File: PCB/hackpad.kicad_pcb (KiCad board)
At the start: 2 copper layers, 93.8 x 82 mm, 36 parts, among them SW11 SW_Push, SW12 SW_Push, SW13 SW_Push, SW14 SW_Push, SW15 SW_Push, SW16 SW_Push, SW17 SW_Push, SW18 SW_Push, SW19 SW_Push, SW4 RotaryEncoder_Switch, U1 MOUDLE-SEEEDUINO-XIAO, U2 ER_OLEDM0.91_1x-I2C

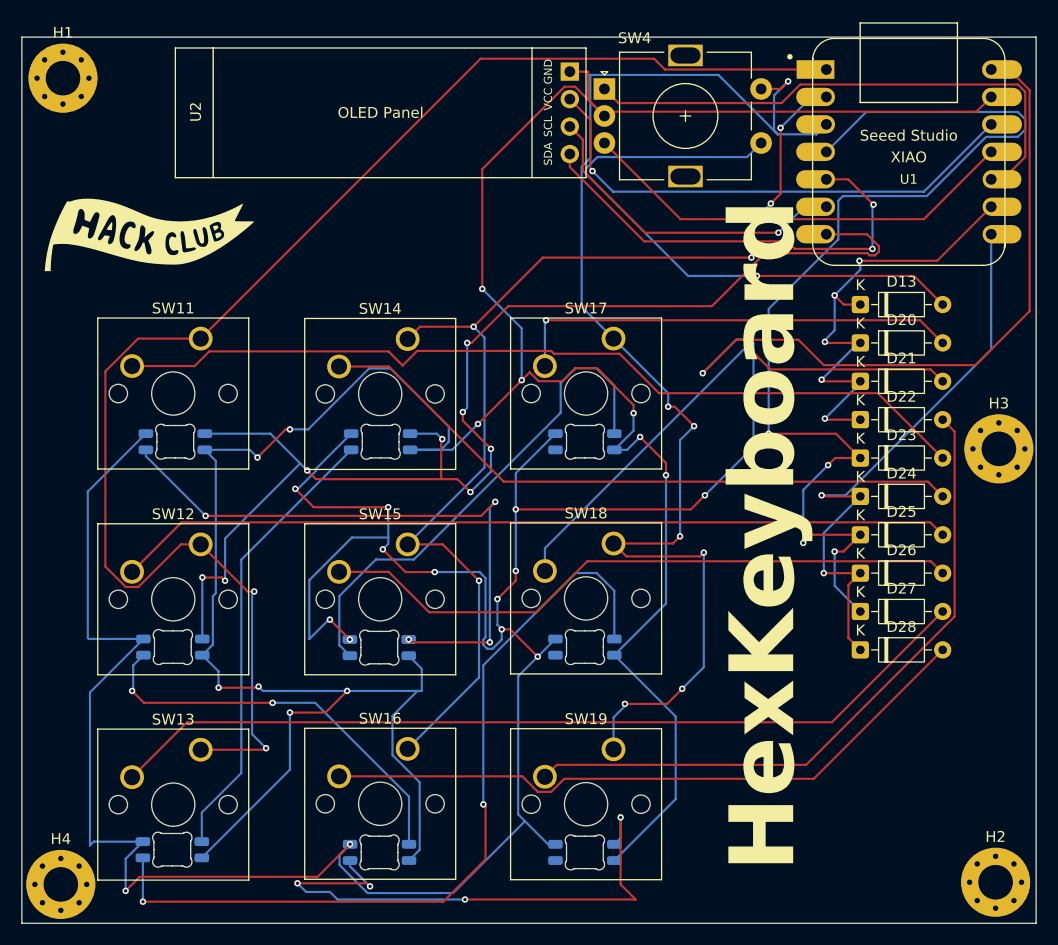
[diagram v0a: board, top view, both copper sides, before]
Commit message: PCB Update
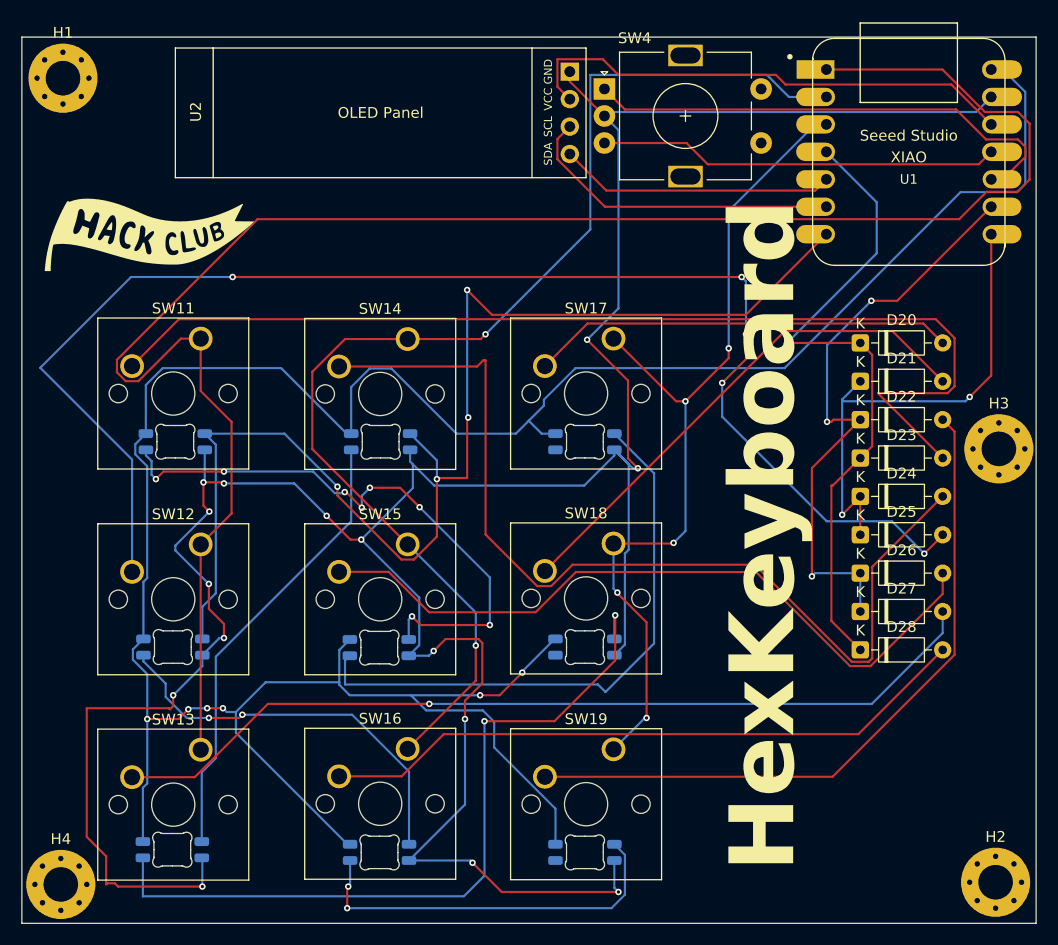
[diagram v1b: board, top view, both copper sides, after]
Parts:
- removed D13: 1N4148, Diode_THT:D_DO-35_SOD27_P7.62mm_Horizontal
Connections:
- D20 pad 1: Net-(D13-K) -> Net-(D20-K)
- D21 pad 1: Net-(D13-K) -> Net-(D21-K)
- D22 pad 1: Net-(D13-K) -> Net-(D22-K)
- D23 pad 1: Net-(D23-K) -> Net-(D20-K)
- D24 pad 1: Net-(D24-K) -> Net-(D21-K)
- D25 pad 1: Net-(D23-K) -> Net-(D21-K)
- D26 pad 1: Net-(D24-K) -> Net-(D22-K)
- D27 pad 1: Net-(D23-K) -> Net-(D22-K)
- D28 pad 1: Net-(D24-K) -> Net-(D20-K)
- SW4 pad S1: Net-(D13-A) -> unconnected-(SW4-PadS1)
- SW4 pad S2: Net-(U1-PA10_A2_D2) -> unconnected-(SW4-PadS2)
- U1 pad 4: Net-(D23-K) -> Net-(D20-K)
- U1 pad 8: Net-(D24-K) -> Net-(D21-K)
- U1 pad 9: Net-(D13-K) -> Net-(D22-K)
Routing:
- net Net-(D23-K): track 101.4 -> 0.00 mm, vias 4 -> 0
- net Net-(D10-VDD): track 310.7 -> 247.6 mm, vias 15 -> 6
- net Net-(D20-K): track 0.00 -> 61.4 mm, vias 0 -> 1
- net Net-(D13-A): track 55.7 -> 0.00 mm, vias 1 -> 0
- net Net-(D24-K): track 55.5 -> 0.00 mm, vias 2 -> 0
- net Net-(D22-K): track 0.00 -> 55.3 mm, vias 0 -> 3
- net Net-(D25-A): track 77.4 -> 131.2 mm, vias 0 -> 5
- net Net-(D21-K): track 0.00 -> 46.8 mm, vias 0 -> 2
- net Net-(D13-K): track 46.0 -> 0.00 mm, vias 5 -> 0
- net Net-(U1-PA10_A2_D2): track 120.5 -> 81.5 mm, vias 7 -> 5
- net Net-(U1-PA02_A0_D0): track 136.4 -> 168.7 mm, vias 2 -> 0
- net Net-(D24-A): track 60.8 -> 90.0 mm
- net Net-(D23-A): track 80.8 -> 98.9 mm
- net Net-(D10-DIN): track 52.8 -> 35.8 mm, vias 4 -> 2
- net Net-(U1-PA8_A4_D4_SDA): track 41.8 -> 25.6 mm, vias 2 -> 0
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
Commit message: Add files via upload
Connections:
- D24 pad 1: Net-(D21-K) -> Net-(D20-K)
- D26 pad 1: Net-(D22-K) -> Net-(D21-K)
- D28 pad 1: Net-(D20-K) -> Net-(D22-K)
- U1 pad 4: Net-(D20-K) -> Net-(D22-K)
- U1 pad 9: Net-(D22-K) -> Net-(D20-K)
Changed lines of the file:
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@@
 			(remove_unused_layers no)
 			(roundrect_rratio 0.15625)
-			(net "Net-(D22-K)")
+			(net "Net-(D21-K)")
 			(pinfunction "K_1")
 			(pintype "passive")
@@
 			(remove_unused_layers no)
 			(roundrect_rratio 0.15625)
-			(net "Net-(D21-K)")
+			(net "Net-(D20-K)")
 			(pinfunction "K_1")
 			(pintype "passive")
@@
 			(remove_unused_layers no)
 			(roundrect_rratio 0.15625)
-			(net "Net-(D20-K)")
+			(net "Net-(D22-K)")
 			(pinfunction "K_1")
 			(pintype "passive")
@@
 			(layers "*.Cu" "*.Mask")
 			(remove_unused_layers no)
-			(net "Net-(D20-K)")
+			(net "Net-(D22-K)")
 			(pinfunction "PA11_A3_D3_4")
 			(pintype "passive")
@@
 			(layers "*.Cu" "*.Mask")
 			(remove_unused_layers no)
-			(net "Net-(D22-K)")
+			(net "Net-(D20-K)")
 			(pinfunction "PA7_A8_D8_SCK_9")
 			(pintype "passive")
